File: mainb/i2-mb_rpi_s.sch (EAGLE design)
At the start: 35 parts, among them IC3 DS1307Z, T1 BC337, T2 BC337, X9 eth (mb->rpi)

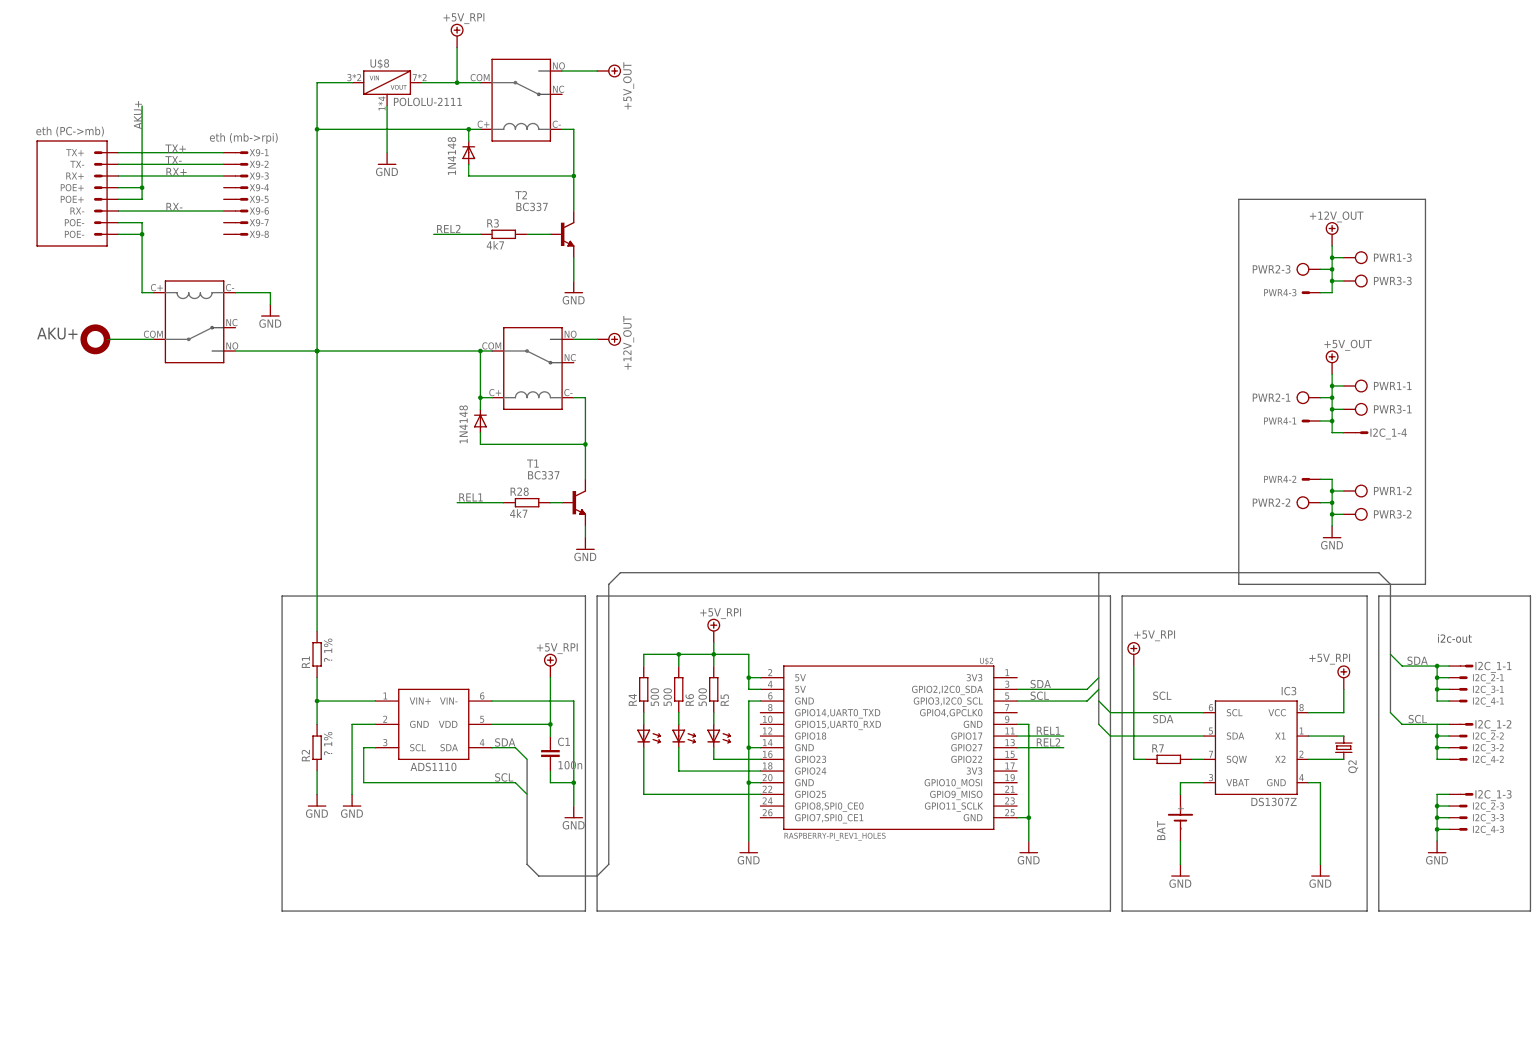
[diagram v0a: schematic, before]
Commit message: 11.12.13 18:50
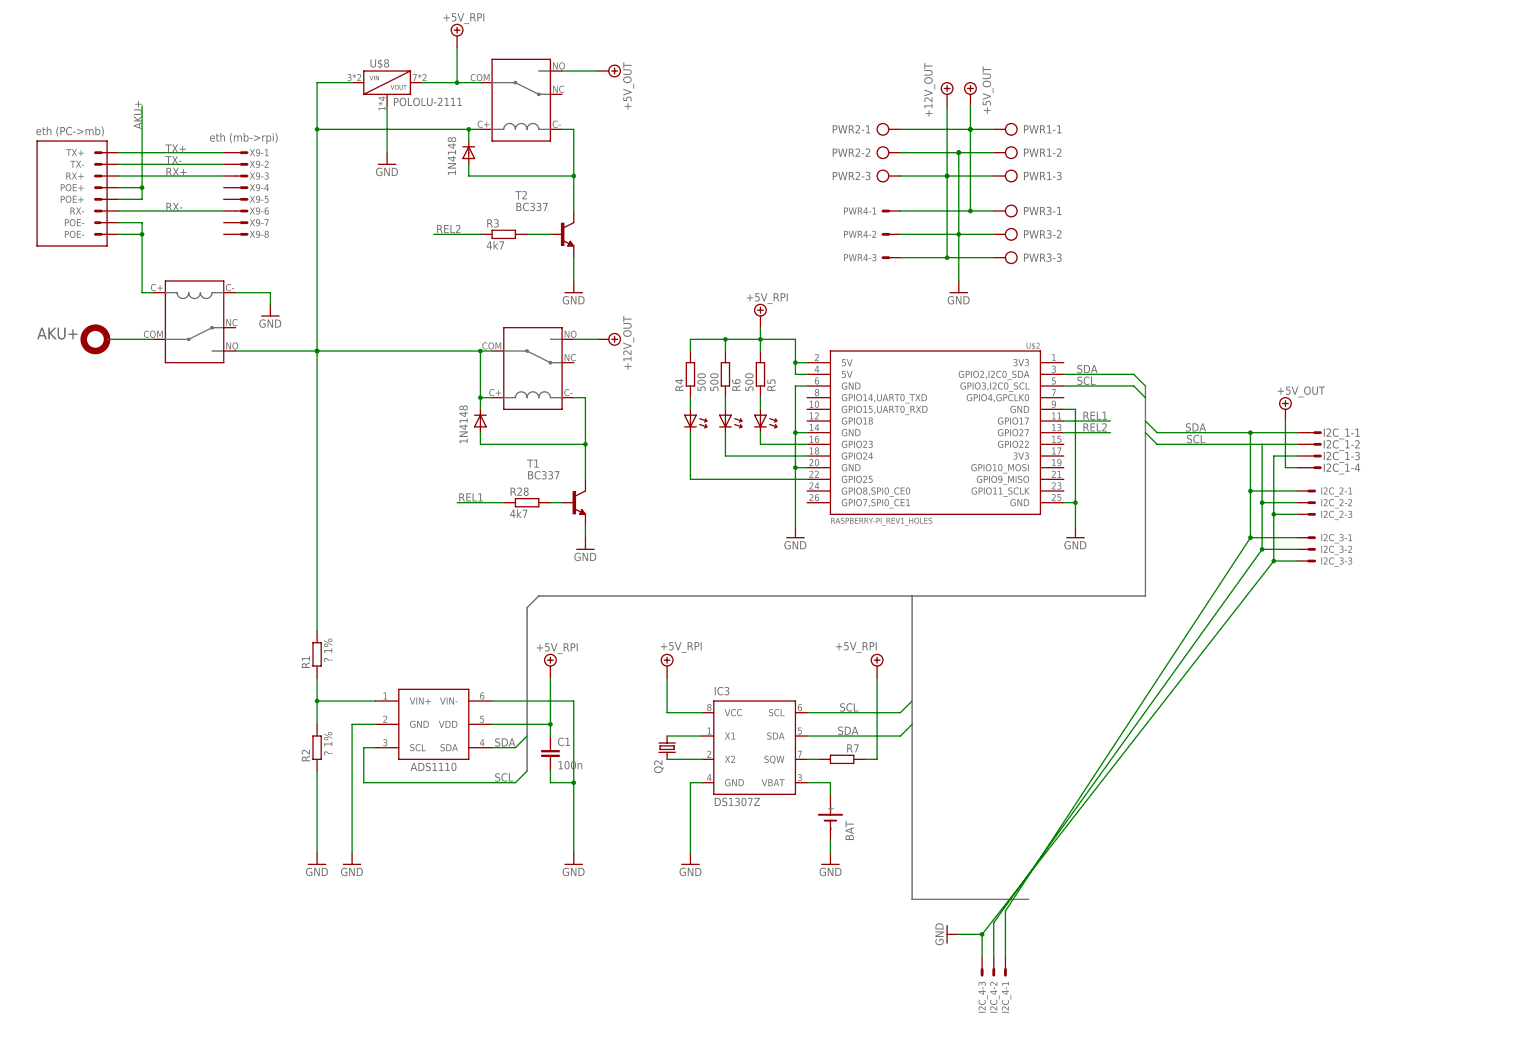
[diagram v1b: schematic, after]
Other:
- note removed: "i2c-out"
- moved on the sheet: BAT, I2C_1-1, I2C_1-2, I2C_1-3, I2C_1-4, I2C_2-1, I2C_2-2, I2C_2-3, I2C_3-1, I2C_3-2, I2C_3-3, I2C_4-1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
